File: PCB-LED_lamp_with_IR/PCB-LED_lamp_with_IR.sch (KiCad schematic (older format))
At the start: 8 parts, among them J1 Conn_01x02_Male, U1 ESP-01v090, U2 AMS1117-3.3

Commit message: lamp
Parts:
- removed J1: Conn_01x02_Male, Connector_PinHeader_2.54mm:PinHeader_1x02_P2.54mm_Vertical, symbol Connector:Conn_01x02_Male
- added U3: TSOP384xx, OptoDevice:Vishay_MINICAST-3Pin, symbol Interface_Optical:TSOP384xx
- U1: symbol ESP8266:ESP-01v090 -> PCB-LED_lamp_with_IR-rescue:ESP-01v090-ESP8266
- U2: footprint TO_SOT_Packages_SMD:SOT-223 -> Package_TO_SOT_SMD:SOT-223-3_TabPin2
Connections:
- net +3V3: now also R2.1, U3.3 (Vs); no longer R2.2
- net GNDREF: now also U3.2 (GND)
- net LEDS1: now reaches R3.2, U1.1 (UTXD)
- net LEDS2: now reaches R1.1, U1.4 (GPIO2)
- net LEDS3: now reaches U1.6 (GPIO0)
- net LEDS3: now also R2.2; no longer R2.1
- net IR: now reaches U1.8 (URXD)
- net IR: now also U3.1 (OUT)
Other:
- moved on the sheet: C1, C2, R1, R2, R3, U2

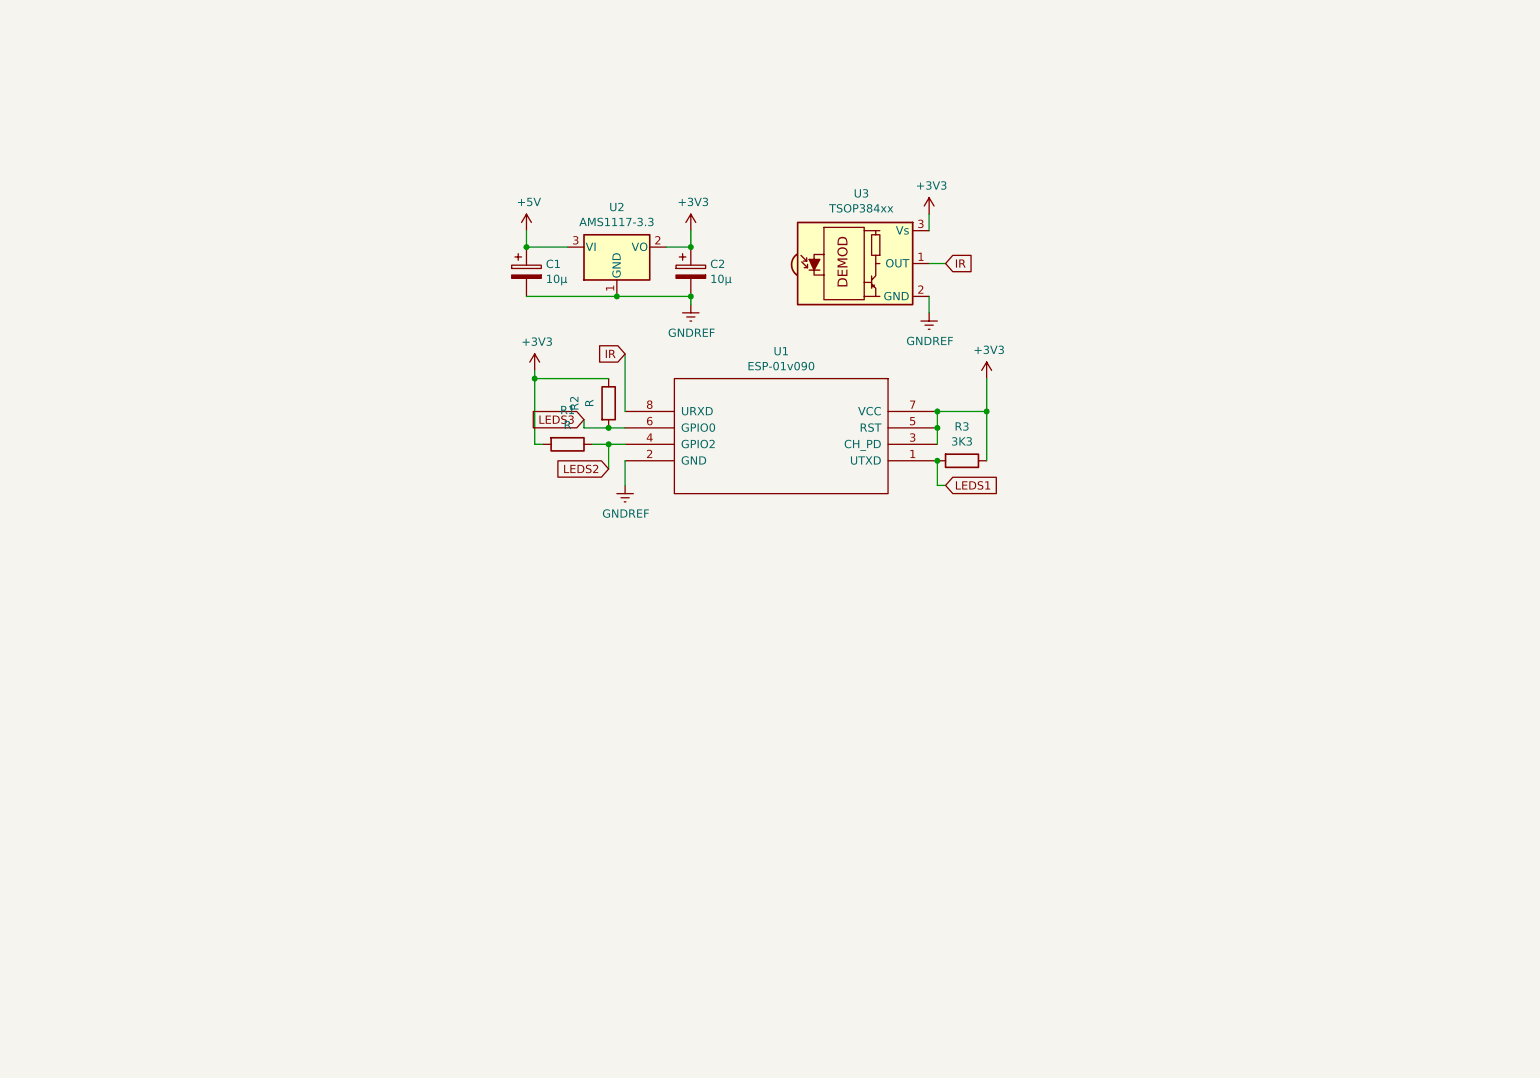
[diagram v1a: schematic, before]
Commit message: leds
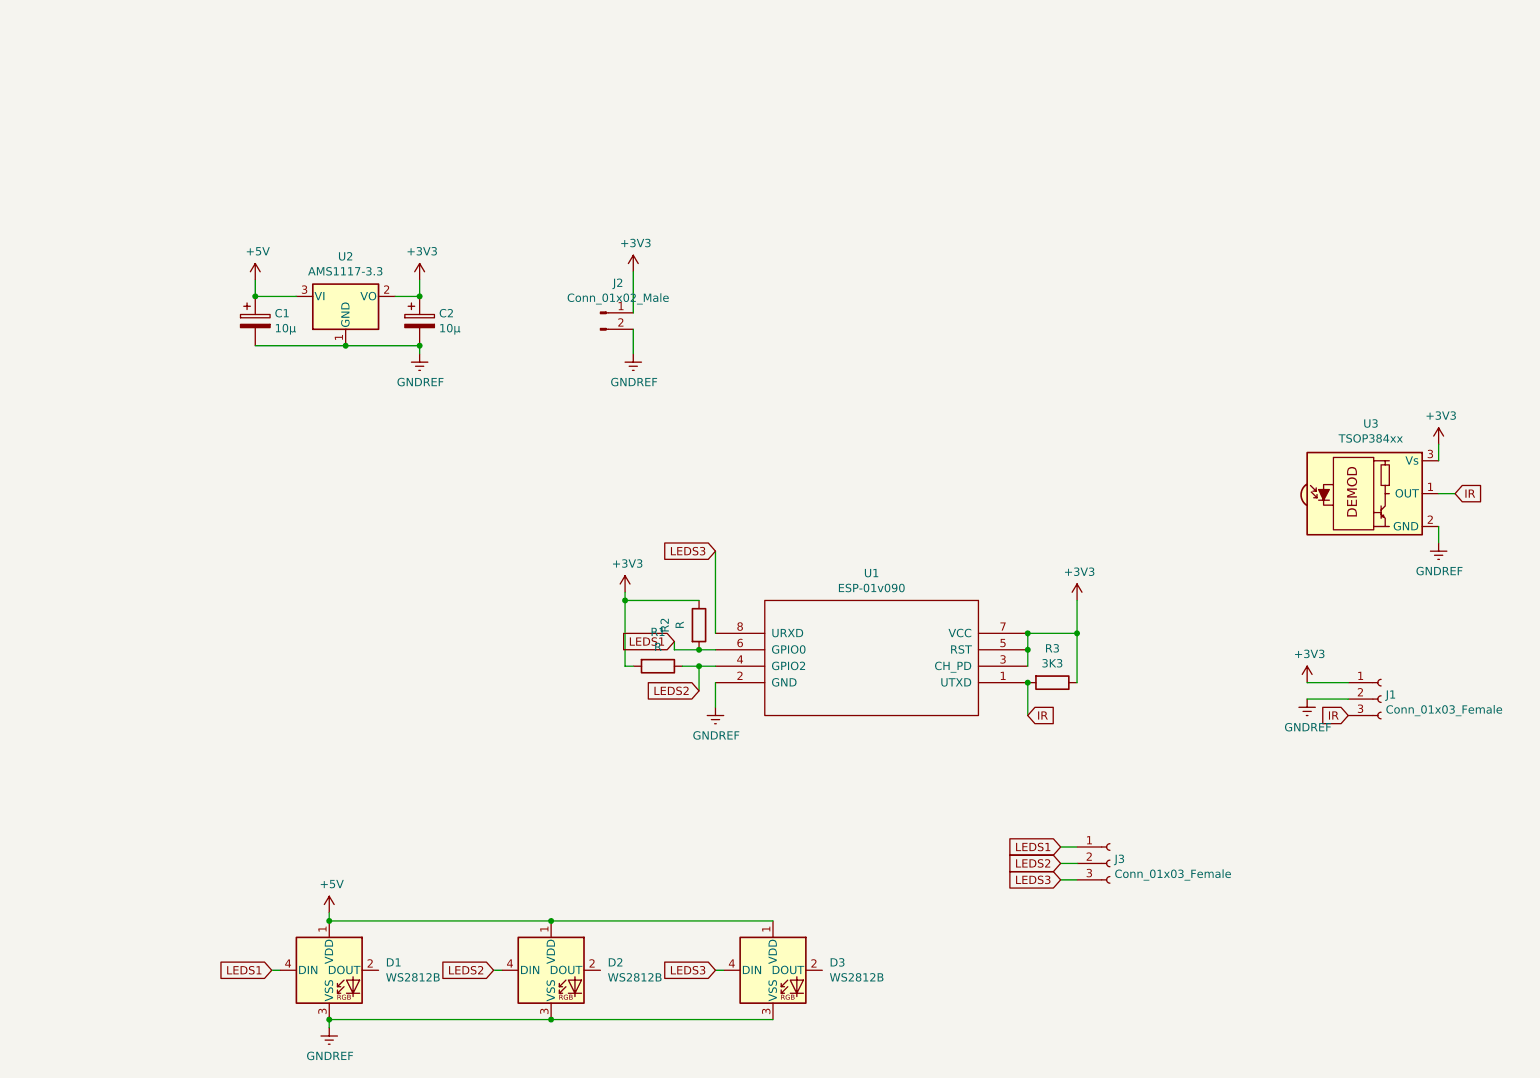
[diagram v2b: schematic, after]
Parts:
- added D1, D2, D3: WS2812B, symbol LED:WS2812B
- added J1: Conn_01x03_Female, Connector_PinSocket_2.54mm:PinSocket_1x03_P2.54mm_Vertical, symbol Connector:Conn_01x03_Female
- added J2: Conn_01x02_Male, Connector_PinSocket_2.54mm:PinSocket_1x02_P2.54mm_Horizontal, symbol Connector:Conn_01x02_Male
- added J3: Conn_01x03_Female, Connector_PinSocket_2.54mm:PinSocket_1x03_P2.54mm_Horizontal, symbol Connector:Conn_01x03_Female
- U3: footprint OptoDevice:Vishay_MINICAST-3Pin -> (none)
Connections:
- net +3V3: now also J1.1 (Pin_1), J2.1 (Pin_1)
- net +5V: now also D1.1 (VDD), D2.1 (VDD), D3.1 (VDD)
- net GNDREF: now also D1.3 (VSS), D2.3 (VSS), D3.3 (VSS), J1.2 (Pin_2), J2.2 (Pin_2)
- net IR: now also R3.2, U1.1 (UTXD), J1.3 (Pin_3); no longer U1.8 (URXD)
- net LEDS1: now also R2.2, U1.6 (GPIO0), D1.4 (DIN), J3.1 (Pin_1); no longer R3.2, U1.1 (UTXD)
- net LEDS2: now also D2.4 (DIN), J3.2 (Pin_2)
- net LEDS3: now also U1.8 (URXD), D3.4 (DIN), J3.3 (Pin_3); no longer R2.2, U1.6 (GPIO0)
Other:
- moved on the sheet: C1, C2, R1, R2, R3, U1, U2, U3
